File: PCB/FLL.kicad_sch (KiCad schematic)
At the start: 11 parts, among them J1 Jack-DC, Q1 2N3819, U1 MCP73831-2-MC, U3 LM317L_SOT-89

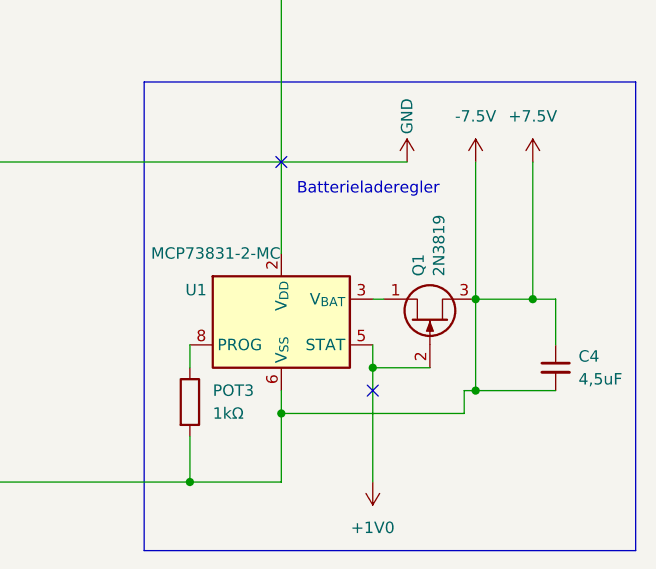
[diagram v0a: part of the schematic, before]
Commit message: chore: Update PCB design configuration and remove unnecessary files
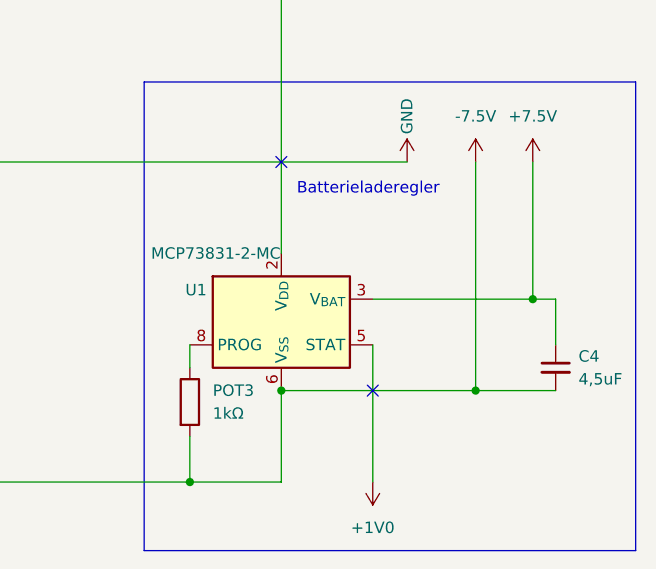
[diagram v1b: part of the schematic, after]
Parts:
- removed Q1: 2N3819, Package_TO_SOT_THT:TO-92, symbol Transistor_FET:2N3819
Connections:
- net +7.5V: now also U1.3 (V_{BAT}), U1.4 (V_{BAT}); no longer C4.2, J1.1, POT3.2, U1.6 (V_{SS})
- new net -7.5V: C4.2, J1.1, POT3.2, U1.6 (V_{SS})
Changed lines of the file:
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@@
-	)
-	(junction
-		(at 200.66 133.35)
-		(diameter 0)
-		(color 0 0 0 0)
 	)
 	(junction
@@
 	)
 	(junction
-		(at 179.07 146.05)
+		(at 179.07 143.51)
 		(diameter 0)
 		(color 0 0 0 0)
@@
 	)
 	(junction
-		(at 189.23 140.97)
+		(at 207.01 133.35)
 		(diameter 0)
 		(color 0 0 0 0)
@@
 	)
 	(junction
-		(at 207.01 133.35)
-		(diameter 0)
-		(color 0 0 0 0)
-	)
-	(junction
 		(at 115.57 97.79)
 		(diameter 0)
@@
 	(wire
 		(pts
-			(xy 189.23 138.43) (xy 189.23 140.97)
-		)
-		(stroke
-			(width 0)
-			(type default)
-		)
-	)
-	(wire
-		(pts
 			(xy 207.01 118.11) (xy 207.01 133.35)
 		)
@@
 	(wire
 		(pts
-			(xy 179.07 153.67) (xy 179.07 146.05)
-		)
-		(stroke
-			(width 0)
-			(type default)
-		)
-	)
-	(wire
-		(pts
 			(xy 140.97 76.2) (xy 115.57 76.2)
 		)
@@
 	(wire
 		(pts
-			(xy 189.23 140.97) (xy 189.23 153.67)
+			(xy 189.23 138.43) (xy 189.23 153.67)
 		)
 		(stroke
@@
 	(wire
 		(pts
+			(xy 189.23 133.35) (xy 207.01 133.35)
+		)
+		(stroke
+			(width 0)
+			(type default)
+		)
+	)
+	(wire
+		(pts
 			(xy 209.55 143.51) (xy 200.66 143.51)
 		)
@@
 	(wire
 		(pts
-			(xy 200.66 118.11) (xy 200.66 133.35)
-		)
-		(stroke
-			(width 0)
-			(type default)
-		)
-	)
-	(wire
-		(pts
-			(xy 179.07 146.05) (xy 179.07 143.51)
+			(xy 200.66 118.11) (xy 200.66 143.51)
+		)
+		(stroke
+			(width 0)
+			(type default)
+		)
+	)
+	(wire
+		(pts
+			(xy 179.07 143.51) (xy 179.07 153.67)
 		)
 		(stroke
@@
 	(wire
 		(pts
-			(xy 200.66 143.51) (xy 199.39 143.51)
-		)
-		(stroke
-			(width 0)
-			(type default)
-		)
-	)
-	(wire
-		(pts
 			(xy 152.4 83.82) (xy 152.4 76.2)
 		)
@@
 	(wire
 		(pts
-			(xy 179.07 146.05) (xy 199.39 146.05)
+			(xy 179.07 143.51) (xy 200.66 143.51)
 		)
 		(stroke
@@
 	(wire
 		(pts
-			(xy 200.66 133.35) (xy 200.66 143.51)
-		)
-		(stroke
-			(width 0)
-			(type default)
-		)
-	)
-	(wire
-		(pts
 			(xy 168.91 153.67) (xy 179.07 153.67)
 		)
@@
 	(wire
 		(pts
-			(xy 200.66 133.35) (xy 207.01 133.35)
-		)
-		(stroke
-			(width 0)
-			(type default)
-		)
-	)
-	(wire
-		(pts
 			(xy 179.07 83.82) (xy 179.07 128.27)
 		)
@@
 	(wire
 		(pts
-			(xy 195.58 140.97) (xy 189.23 140.97)
-		)
-		(stroke
-			(width 0)
-			(type default)
-		)
-	)
-	(wire
-		(pts
 			(xy 142.24 83.82) (xy 142.24 86.36)
 		)
@@
 	(wire
 		(pts
-			(xy 199.39 146.05) (xy 199.39 143.51)
-		)
-		(stroke
-			(width 0)
-			(type default)
-		)
-	)
-	(wire
-		(pts
 			(xy 116.84 83.82) (xy 115.57 83.82)
 		)
@@
 		(pts
 			(xy 132.08 93.98) (xy 132.08 97.79)
-		)
-		(stroke
-			(width 0)
-			(type default)
-		)
-	)
-	(wire
-		(pts
-			(xy 190.5 133.35) (xy 189.23 133.35)
 		)
 		(stroke
@@
 					(unit 1)
 				)
-			)
-		)
-	)
-	(symbol
-		(lib_id "Transistor_FET:2N3819")
-		(at 195.58 135.89 90)
-		(unit 1)
-		(exclude_from_sim no)
-		(in_bom yes)
-		(on_board yes)
-		(dnp no)
-		(property "Reference" "Q1"
-			(at 194.3099 130.81 0)
-			(effects
-				(font
-					(size 1.27 1.27)
-				)
-				(justify left)
-			)
-		)
-		(property "Value" "2N3819"
-			(at 196.596 130.81 0)
-			(effects
-				(font
-					(size 1.27 1.27)
-				)
-				(justify left)
-			)
-		)
-		(property "Footprint" "Package_TO_SOT_THT:TO-92"
-			(at 197.485 130.81 0)
-			(effects
-				(font
-					(size 1.27 1.27)
-					(italic yes)
-				)
-				(justify left)
-				(hide yes)
-			)
-		)
-		(property "Datasheet" "https://my.centralsemi.com/datasheets/2N3819.PDF"
-			(at 199.39 130.81 0)
-			(effects
-				(font
-					(size 1.27 1.27)
-				)
-				(justify left)
-				(hide yes)
-			)
-		)
-		(property "Description" "20mA Id, 25V Vgs, N-Channel JFET Transistor, TO-92"
-			(at 195.58 135.89 0)
-			(effects
-				(font
-					(size 1.27 1.27)
-				)
-				(hide yes)
-			)
-		)
-		(pin "1"
-		)
-		(pin "2"
-		)
-		(pin "3"
-		)
-		(instances
-			(project ""
-				(path "/eebf961a-9e34-427c-a1d5-e0dfc5b48cc6"
-					(reference "Q1")
-					(unit 1)
-				)
